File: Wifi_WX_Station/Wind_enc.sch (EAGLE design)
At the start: 9 parts, among them U1 AS5030

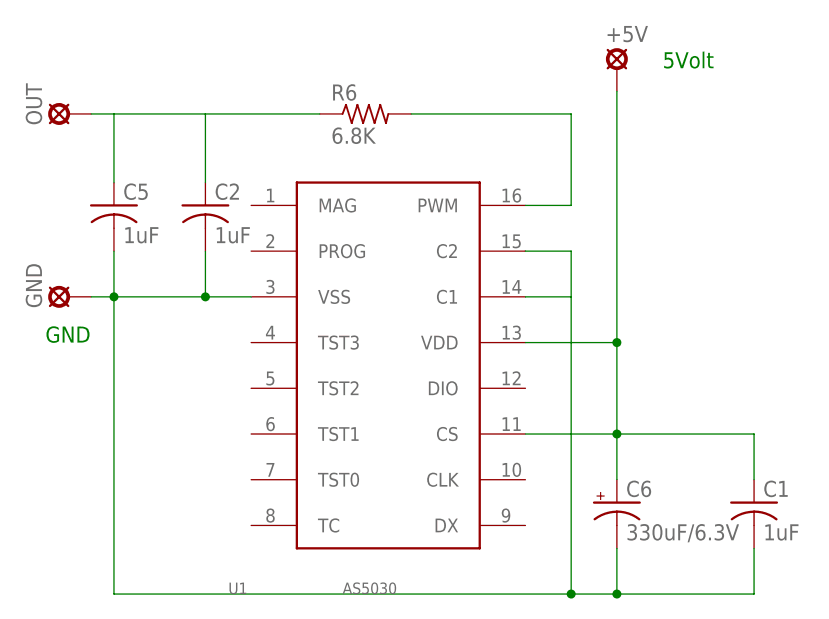
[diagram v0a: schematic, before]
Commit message: updated BOM with all prices- As Checked in to BATCH PCB
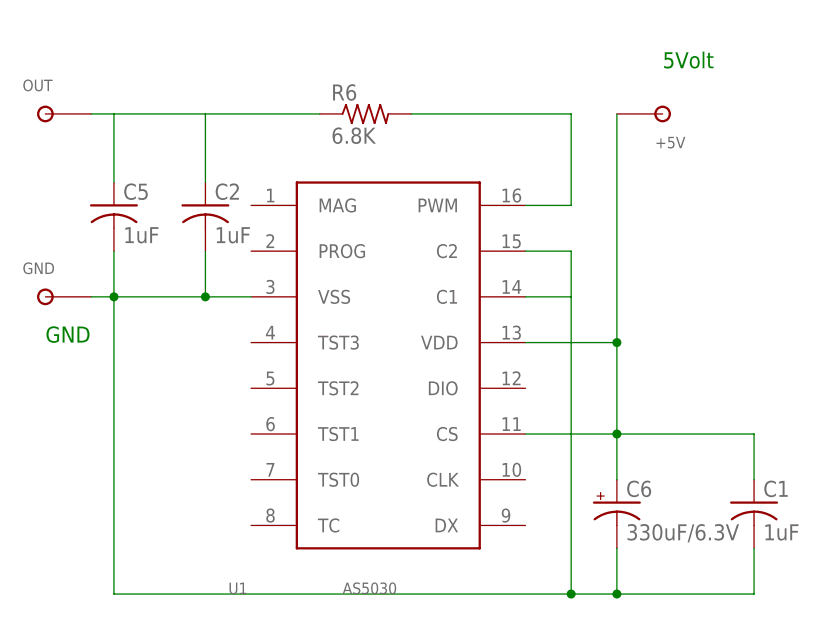
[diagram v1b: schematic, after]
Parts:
- +5V, GND, OUT: value LSP10 -> TPSOL; device solpad:LSP10 -> wifi_WX:TPSOL
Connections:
- net N$1: now also +5V.P$1; no longer +5V.MP
- net N$2: now also GND.P$1; no longer GND.MP
- net N$22: now also OUT.P$1; no longer OUT.MP
